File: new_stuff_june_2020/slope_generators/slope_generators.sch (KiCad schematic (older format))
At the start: 0 parts

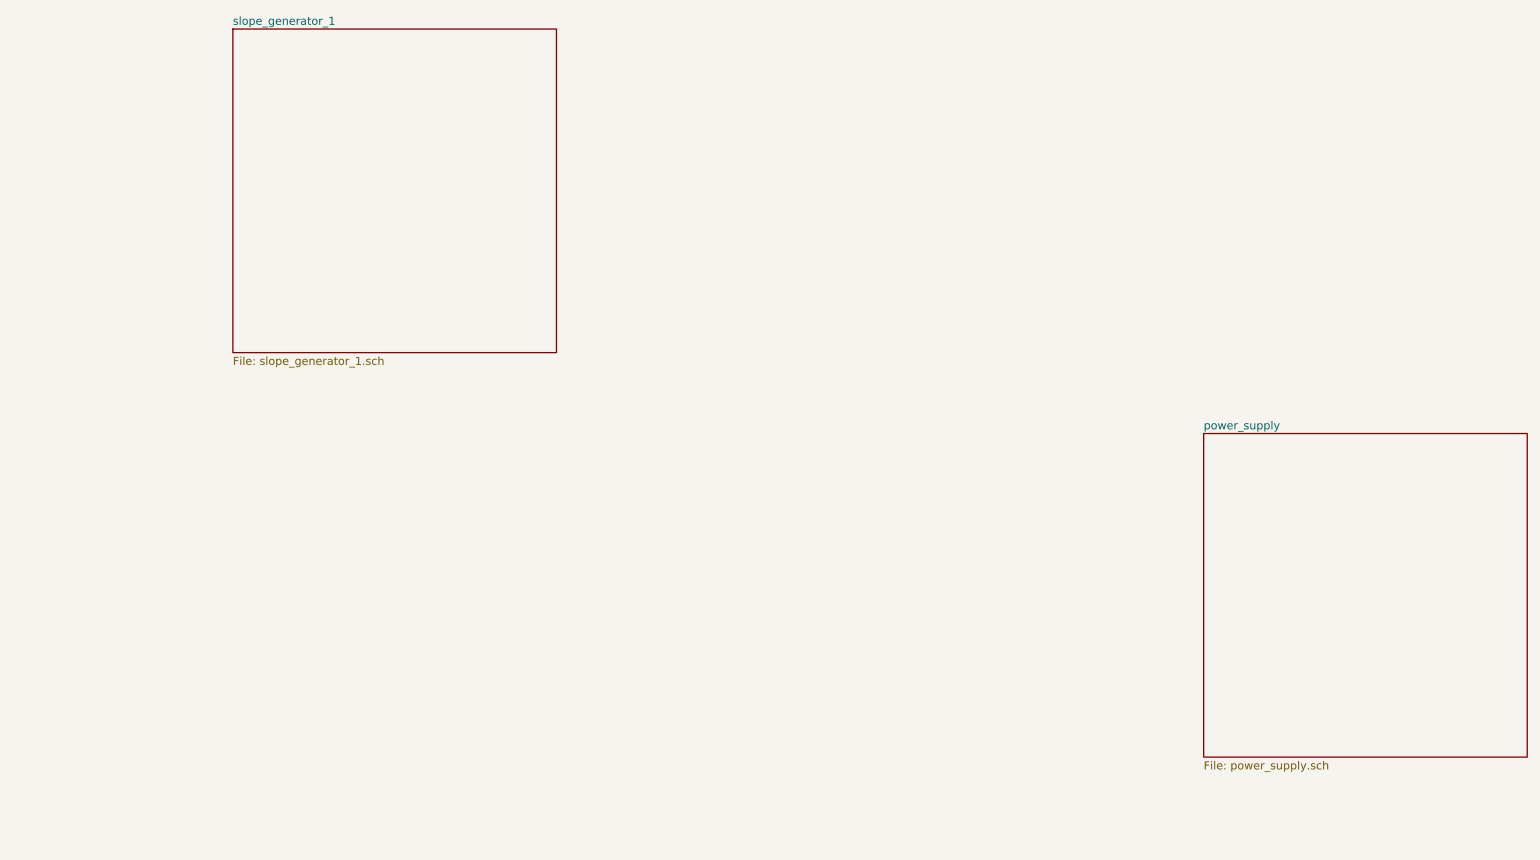
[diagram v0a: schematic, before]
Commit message: slope gen progress, misc cleanup
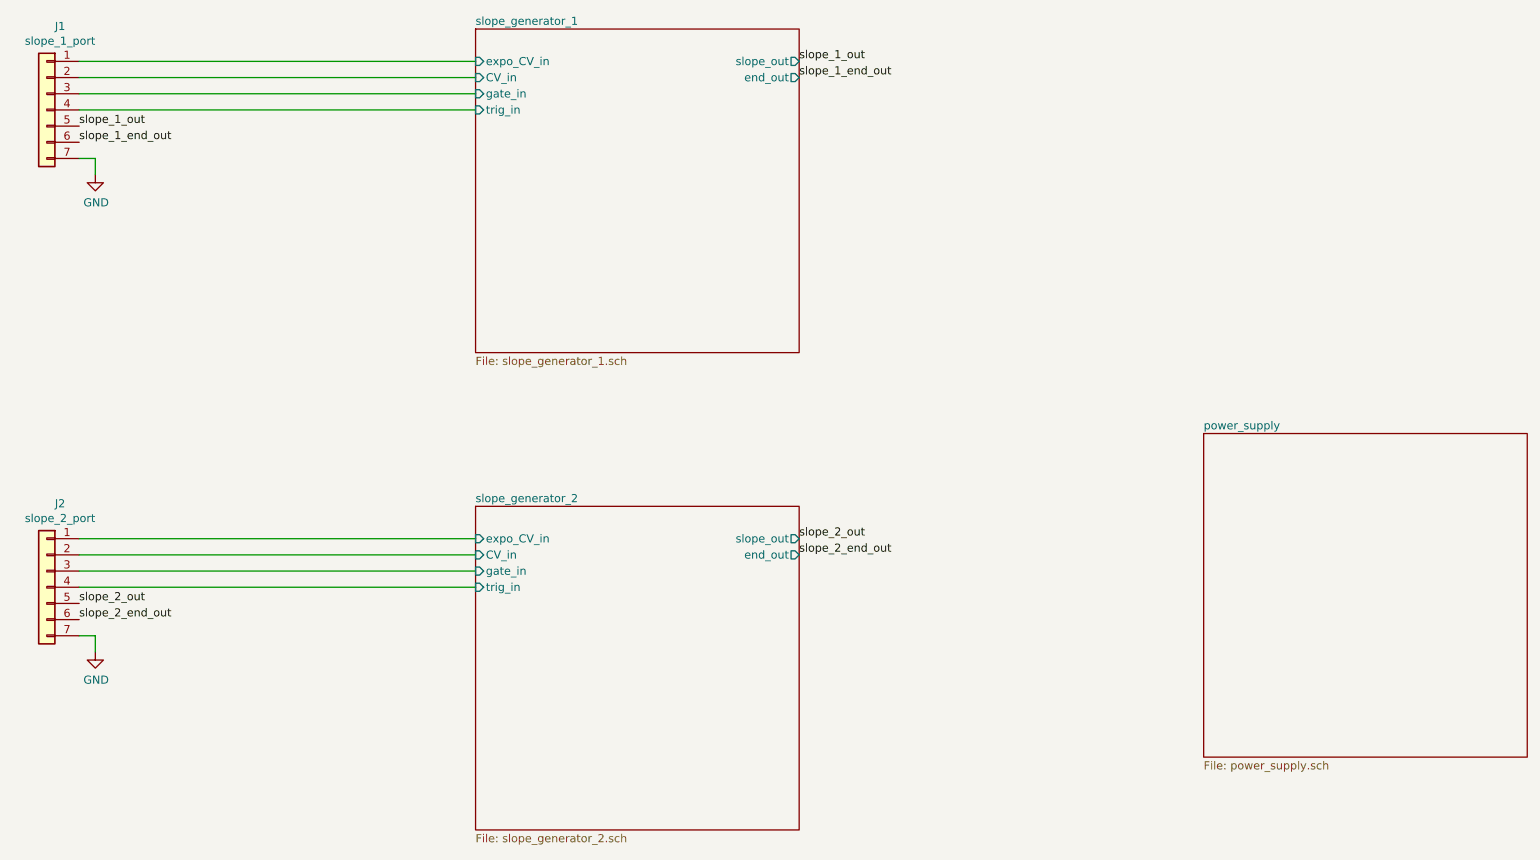
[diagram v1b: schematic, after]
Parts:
- added J1: slope_1_port, Connector_PinHeader_2.54mm:PinHeader_1x07_P2.54mm_Vertical, symbol Connector_Generic:Conn_01x07
- added J2: slope_2_port, Connector_PinHeader_2.54mm:PinHeader_1x07_P2.54mm_Vertical, symbol Connector_Generic:Conn_01x07
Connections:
- new net GND: J1.7 (Pin_7), J2.7 (Pin_7)
- new net slope_1_end_out: J1.6 (Pin_6)
- new net slope_1_out: J1.5 (Pin_5)
- new net slope_2_end_out: J2.6 (Pin_6)
- new net slope_2_out: J2.5 (Pin_5)
- new net slope_generator_1/CV_in: J1.2 (Pin_2)
- new net slope_generator_1/expo_CV_in: J1.1 (Pin_1)
- new net slope_generator_1/gate_in: J1.3 (Pin_3)
- new net slope_generator_1/trig_in: J1.4 (Pin_4)
- new net slope_generator_2/CV_in: J2.2 (Pin_2)
- new net slope_generator_2/expo_CV_in: J2.1 (Pin_1)
- new net slope_generator_2/gate_in: J2.3 (Pin_3)
- new net slope_generator_2/trig_in: J2.4 (Pin_4)
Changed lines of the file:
@@
 $Descr A4 11693 8268
 encoding utf-8
-Sheet 1 3
+Sheet 1 4
 Title ""
 Date ""
@@
 $EndDescr
 $Sheet
-S 2500 1500 2000 2000
+S 4000 1500 2000 2000
 U 5EEA5DFE
 F0 "slope_generator_1" 50
 F1 "slope_generator_1.sch" 50
+F2 "expo_CV_in" I L 4000 1700 50
+F3 "gate_in" I L 4000 1900 50
+F4 "trig_in" I L 4000 2000 50
+F5 "slope_out" O R 6000 1700 50
+F6 "end_out" O R 6000 1800 50
+F7 "CV_in" I L 4000 1800 50
 $EndSheet
 $Sheet
@@
 F1 "power_supply.sch" 50
 $EndSheet
+$Sheet
+S 4000 4450 2000 2000
+U 5F422028
+F0 "slope_generator_2" 50
+F1 "slope_generator_2.sch" 50
+F2 "expo_CV_in" I L 4000 4650 50
+F3 "gate_in" I L 4000 4850 50
+F4 "trig_in" I L 4000 4950 50
+F5 "slope_out" O R 6000 4650 50
+F6 "end_out" O R 6000 4750 50
+F7 "CV_in" I L 4000 4750 50
+$EndSheet
+$Comp
+L Connector_Generic:Conn_01x07 J1
+U 1 1 5F486705
+P 1350 2000
+F 0 "J1" H 1268 2517 50  0000 C CNN
+F 1 "slope_1_port" H 1268 2426 50  0000 C CNN
+F 2 "Connector_PinHeader_2.54mm:PinHeader_1x07_P2.54mm_Vertical" H 1350 2000 50  0001 C CNN
+F 3 "~" H 1350 2000 50  0001 C CNN
+	1    1350 2000
+	-1   0    0    -1
+$EndComp
+Wire Wire Line
+	1550 1700 4000 1700
+Wire Wire Line
+	1550 1800 4000 1800
+Wire Wire Line
+	1550 1900 4000 1900
+Wire Wire Line
+	1550 2000 4000 2000
+$Comp
+L power:GND #PWR070
+U 1 1 5F487E68
+P 1650 2400
+F 0 "#PWR070" H 1650 2150 50  0001 C CNN
+F 1 "GND" H 1655 2227 50  0000 C CNN
+F 2 "" H 1650 2400 50  0001 C CNN
+F 3 "" H 1650 2400 50  0001 C CNN
+	1    1650 2400
+	1    0    0    -1
+$EndComp
+Wire Wire Line
+	1650 2400 1650 2300
+Wire Wire Line
+	1650 2300 1550 2300
+$Comp
+L Connector_Generic:Conn_01x07 J2
+U 1 1 5F488F2D
+P 1350 4950
+F 0 "J2" H 1268 5467 50  0000 C CNN
+F 1 "slope_2_port" H 1268 5376 50  0000 C CNN
+F 2 "Connector_PinHeader_2.54mm:PinHeader_1x07_P2.54mm_Vertical" H 1350 4950 50  0001 C CNN
+F 3 "~" H 1350 4950 50  0001 C CNN
+	1    1350 4950
+	-1   0    0    -1
+$EndComp
+Wire Wire Line
+	1550 4650 4000 4650
+Wire Wire Line
+	1550 4750 4000 4750
+Wire Wire Line
+	1550 4850 4000 4850
+Wire Wire Line
+	1550 4950 4000 4950
+$Comp
+L power:GND #PWR071
+U 1 1 5F488F37
+P 1650 5350
+F 0 "#PWR071" H 1650 5100 50  0001 C CNN
+F 1 "GND" H 1655 5177 50  0000 C CNN
+F 2 "" H 1650 5350 50  0001 C CNN
+F 3 "" H 1650 5350 50  0001 C CNN
+	1    1650 5350
+	1    0    0    -1
+$EndComp
+Wire Wire Line
+	1650 5350 1650 5250
+Wire Wire Line
+	1650 5250 1550 5250
+Text Label 1550 5050 0    50   ~ 0
+slope_2_out
+Text Label 1550 5150 0    50   ~ 0
+slope_2_end_out
+Text Label 6000 4650 0    50   ~ 0
+slope_2_out
+Text Label 6000 4750 0    50   ~ 0
+slope_2_end_out
+Text Label 6000 1700 0    50   ~ 0
+slope_1_out
+Text Label 6000 1800 0    50   ~ 0
+slope_1_end_out
+Text Label 1550 2100 0    50   ~ 0
+slope_1_out
+Text Label 1550 2200 0    50   ~ 0
+slope_1_end_out
 $EndSCHEMATC
